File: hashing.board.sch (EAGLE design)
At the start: 145 parts, among them U1 ASIC-1, U10 EPM570GT100C5N, U11 BFL-ASIC-1, U2 ASIC-1, U3 ASIC-1, U4 ASIC-1, U5 ASIC-1, U6 ASIC-1, U7 ASIC-1, U8 ASIC-1, U9 AT32UC3A1256-AUT, X1 5566-8, X2 5566-8, X3 MINI-USB-32005-301, X4 22-23-2031

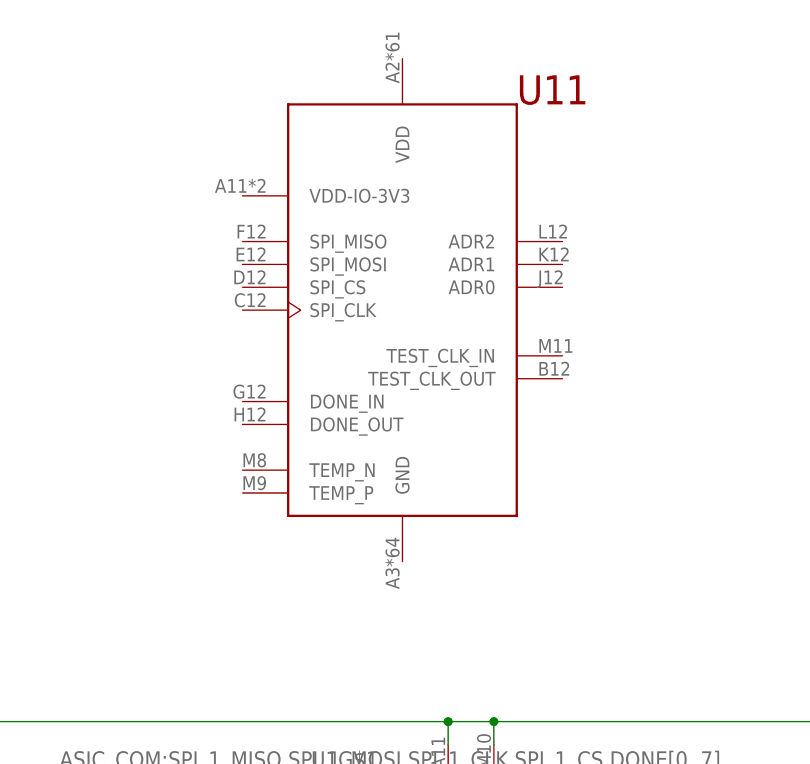
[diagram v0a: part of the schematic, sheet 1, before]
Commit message: broken
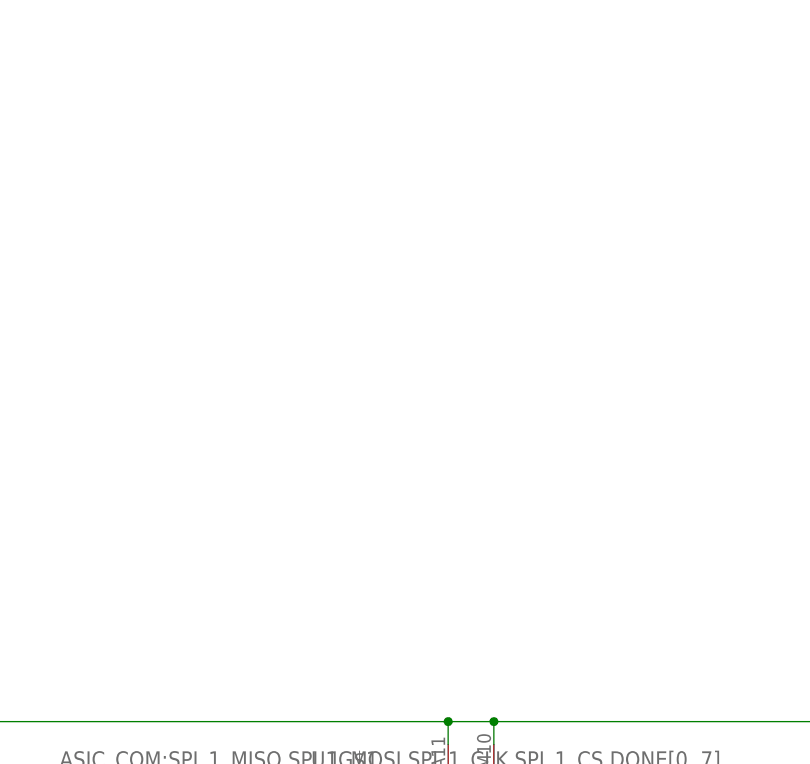
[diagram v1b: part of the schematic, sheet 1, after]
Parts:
- removed U11: BFL-ASIC-1, BFL.new:BFL-ASIC-1
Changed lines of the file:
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@@
 <grid distance="0.1" unitdist="inch" unit="inch" style="lines" multiple="1" display="no" altdistance="0.01" altunitdist="inch" altunit="inch"/>
 <layers>
-<layer number="1" name="Top" color="4" fill="1" visible="no" active="no"/>
-<layer number="2" name="Route2" color="1" fill="3" visible="no" active="no"/>
-<layer number="3" name="Route3" color="4" fill="3" visible="no" active="no"/>
-<layer number="14" name="Route14" color="1" fill="6" visible="no" active="no"/>
-<layer number="15" name="Route15" color="4" fill="6" visible="no" active="no"/>
-<layer number="16" name="Bottom" color="1" fill="1" visible="no" active="no"/>
-<layer number="17" name="Pads" color="2" fill="1" visible="no" active="no"/>
-<layer number="18" name="Vias" color="2" fill="1" visible="no" active="no"/>
-<layer number="19" name="Unrouted" color="6" fill="1" visible="no" active="no"/>
-<layer number="20" name="Dimension" color="15" fill="1" visible="no" active="no"/>
-<layer number="21" name="tPlace" color="7" fill="1" visible="no" active="no"/>
-<layer number="22" name="bPlace" color="7" fill="1" visible="no" active="no"/>
-<layer number="23" name="tOrigins" color="15" fill="1" visible="no" active="no"/>
-<layer number="24" name="bOrigins" color="15" fill="1" visible="no" active="no"/>
-<layer number="25" name="tNames" color="7" fill="1" visible="no" active="no"/>
-<layer number="26" name="bNames" color="7" fill="1" visible="no" active="no"/>
-<layer number="27" name="tValues" color="7" fill="1" visible="no" active="no"/>
-<layer number="28" name="bValues" color="7" fill="1" visible="no" active="no"/>
+<layer number="1" name="Top" color="4" fill="1" visible="yes" active="no"/>
+<layer number="2" name="Route2" color="1" fill="3" visible="yes" active="no"/>
+<layer number="3" name="Route3" color="4" fill="3" visible="yes" active="no"/>
+<layer number="14" name="Route14" color="1" fill="6" visible="yes" active="no"/>
+<layer number="15" name="Route15" color="4" fill="6" visible="yes" active="no"/>
+<layer number="16" name="Bottom" color="1" fill="1" visible="yes" active="no"/>
+<layer number="17" name="Pads" color="2" fill="1" visible="yes" active="no"/>
+<layer number="18" name="Vias" color="2" fill="1" visible="yes" active="no"/>
+<layer number="19" name="Unrouted" color="6" fill="1" visible="yes" active="no"/>
+<layer number="20" name="Dimension" color="15" fill="1" visible="yes" active="no"/>
+<layer number="21" name="tPlace" color="7" fill="1" visible="yes" active="no"/>
+<layer number="22" name="bPlace" color="7" fill="1" visible="yes" active="no"/>
+<layer number="23" name="tOrigins" color="15" fill="1" visible="yes" active="no"/>
+<layer number="24" name="bOrigins" color="15" fill="1" visible="yes" active="no"/>
+<layer number="25" name="tNames" color="7" fill="1" visible="yes" active="no"/>
+<layer number="26" name="bNames" color="7" fill="1" visible="yes" active="no"/>
+<layer number="27" name="tValues" color="7" fill="1" visible="yes" active="no"/>
+<layer number="28" name="bValues" color="7" fill="1" visible="yes" active="no"/>
 <layer number="29" name="tStop" color="7" fill="3" visible="no" active="no"/>
 <layer number="30" name="bStop" color="7" fill="6" visible="no" active="no"/>
@@
 <layer number="35" name="tGlue" color="7" fill="4" visible="no" active="no"/>
 <layer number="36" name="bGlue" color="7" fill="5" visible="no" active="no"/>
-<layer number="37" name="tTest" color="7" fill="1" visible="no" active="no"/>
-<layer number="38" name="bTest" color="7" fill="1" visible="no" active="no"/>
+<layer number="37" name="tTest" color="7" fill="1" visible="yes" active="no"/>
+<layer number="38" name="bTest" color="7" fill="1" visible="yes" active="no"/>
 <layer number="39" name="tKeepout" color="4" fill="11" visible="no" active="no"/>
 <layer number="40" name="bKeepout" color="1" fill="11" visible="no" active="no"/>
@@
 <layer number="44" name="Drills" color="7" fill="1" visible="no" active="no"/>
 <layer number="45" name="Holes" color="7" fill="1" visible="no" active="no"/>
-<layer number="46" name="Milling" color="3" fill="1" visible="no" active="no"/>
-<layer number="47" name="Measures" color="7" fill="1" visible="no" active="no"/>
-<layer number="48" name="Document" color="7" fill="1" visible="no" active="no"/>
-<layer number="49" name="Reference" color="7" fill="1" visible="no" active="no"/>
-<layer number="51" name="tDocu" color="7" fill="1" visible="no" active="no"/>
-<layer number="52" name="bDocu" color="7" fill="1" visible="no" active="no"/>
+<layer number="46" name="Milling" color="3" fill="1" visible="yes" active="no"/>
+<layer number="47" name="Measures" color="7" fill="1" visible="yes" active="no"/>
+<layer number="48" name="Document" color="7" fill="1" visible="yes" active="no"/>
+<layer number="49" name="Reference" color="7" fill="1" visible="yes" active="no"/>
+<layer number="51" name="tDocu" color="7" fill="1" visible="yes" active="no"/>
+<layer number="52" name="bDocu" color="7" fill="1" visible="yes" active="no"/>
 <layer number="91" name="Nets" color="2" fill="1" visible="yes" active="yes"/>
 <layer number="92" name="Busses" color="1" fill="1" visible="yes" active="yes"/>
@@
 <part name="CA7" library="casey's_custom_stuff" deviceset="BFL-BGA-144-SPC" device=""/>
 <part name="CA8" library="casey's_custom_stuff" deviceset="BFL-BGA-144-SPC" device=""/>
-<part name="U11" library="BFL.new" deviceset="BFL-ASIC-1" device=""/>
 </parts>
 <sheets>
@@
 <instance part="FRAME2" gate="G$1" x="0" y="0"/>
 <instance part="FRAME2" gate="G$2" x="325.12" y="0"/>
-<instance part="U11" gate="G$1" x="139.7" y="213.36"/>
 </instances>
 <busses>
